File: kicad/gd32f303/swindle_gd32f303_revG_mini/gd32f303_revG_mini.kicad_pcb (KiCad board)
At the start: 2 copper layers, 39.3 x 30.1 mm, 54 parts, among them J1 Debug port, J2 Debug port, J3 USB, J40 J40, J7 Conn_01x05_Pin, Q1 DMG2302U, U1 GD32F303, U5 LM1117-3.3, Y2 8Mhz

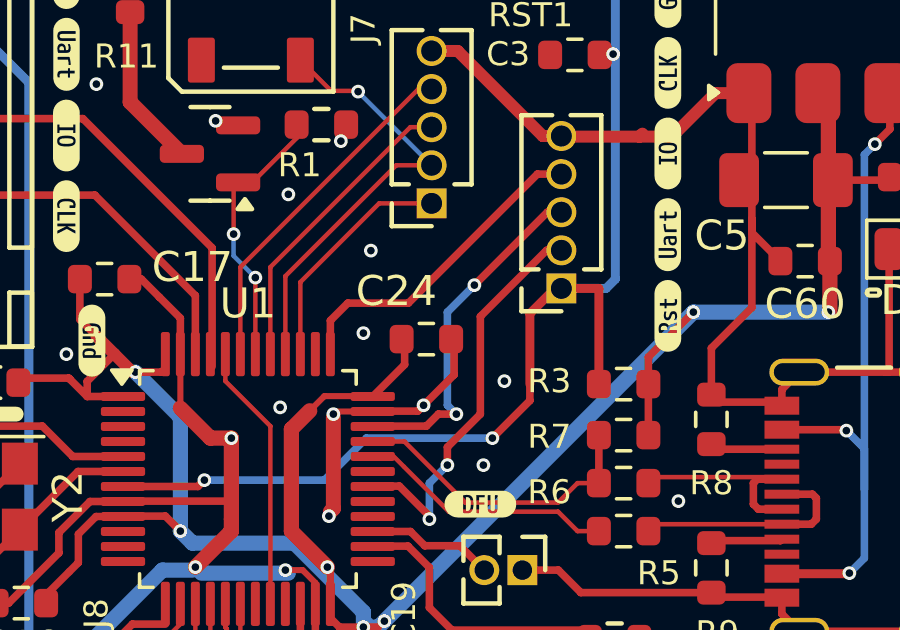
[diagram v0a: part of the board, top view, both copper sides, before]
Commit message: kicad : g32, cosmetic
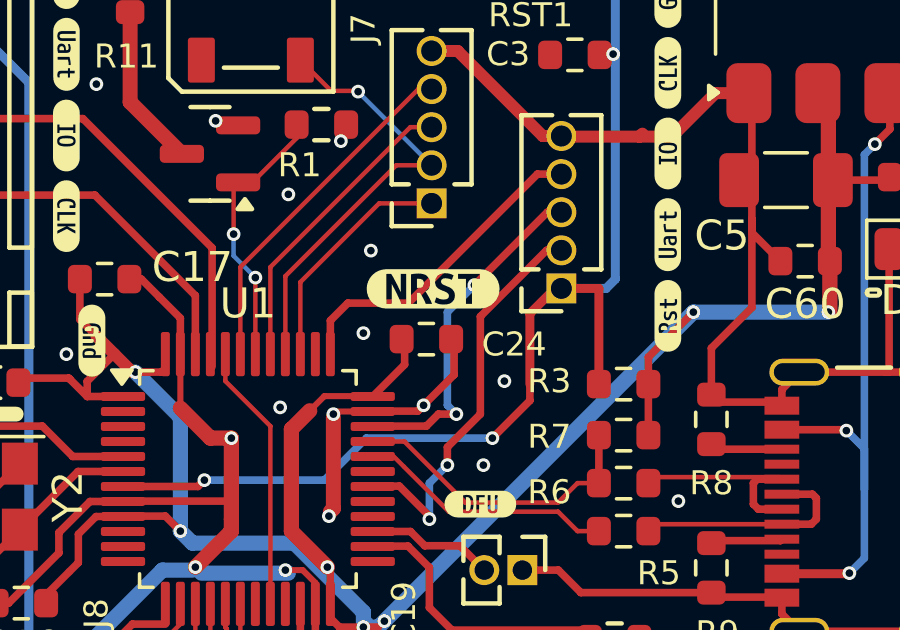
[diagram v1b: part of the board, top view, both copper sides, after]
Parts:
- added kibuzzard-68AB27BD: G***, kibuzzard-68AB27BD, F.Cu at (136.4, 84.6)
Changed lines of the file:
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@@
+		)
+	)
+	(footprint "kibuzzard-68AB27BD"
+		(layer "F.Cu")
+		(at 136.425 84.625)
+		(descr "Generated with KiBuzzard")
+		(tags "kb_params=eyJBbGlnbm1lbnRDaG9pY2UiOiAiQ2VudGVyIiwgIkNhcExlZnRDaG9pY2UiOiAiKCIsICJDYXBSaWdodENob2ljZSI6ICIpIiwgIkZvbnRDb21ib0JveCI6ICJVYnVudHVNb25vLUIiLCAiSGVpZ2h0Q3RybCI6IDEuMCwgIkxheWVyQ29tYm9Cb3giOiAiRi5TaWxrUyIsICJMaW5lU3BhY2luZ0N0cmwiOiAwLjYsICJNdWx0aUxpbmVUZXh0IjogIk5SU1QiLCAiUGFkZGluZ0JvdHRvbUN0cmwiOiAxLjAsICJQYWRkaW5nTGVmdEN0cmwiOiAwLjAsICJQYWRkaW5nUmlnaHRDdHJsIjogMC4wLCAiUGFkZGluZ1RvcEN0cmwiOiAxLjAsICJXaWR0aEN0cmwiOiAyLjgsICJhZHZhbmNlZENoZWNrYm94IjogZmFsc2UsICJpbmxpbmVGb3JtYXRUZXh0Ym94IjogZmFsc2UsICJsaW5lb3ZlclN0eWxlQ2hvaWNlIjogIlNxdWFyZSIsICJsaW5lb3ZlclRoaWNrbmVzc0N0cmwiOiAxfQ==")
+		(property "Reference" "kibuzzard-68AB27BD"
+			(at 0 -3.704435 0)
+			(layer "F.SilkS")
+			(hide yes)
+			(effects
+				(font
+					(size 0.001 0.001)
+				)
+			)
+		)
+		(property "Value" "G***"
+			(at 0 3.704435 0)
+			(layer "F.SilkS")
+			(hide yes)
+			(effects
+				(font
+					(size 0.001 0.001)
+				)
+			)
+		)
+		(property "Footprint" ""
+			(at 0 0 0)
+			(layer "F.Fab")
+			(hide yes)
+			(effects
+				(font
+					(size 1.27 1.27)
+					(thickness 0.15)
+				)
+			)
+		)
+		(property "Datasheet" ""
+			(at 0 0 0)
+			(layer "F.Fab")
+			(hide yes)
+			(effects
+				(font
+					(size 1.27 1.27)
+					(thickness 0.15)
+				)
+			)
+		)
+		(property "Description" ""
+			(at 0 0 0)
+			(layer "F.Fab")
+			(hide yes)
+			(effects
+				(font
+					(size 1.27 1.27)
+					(thickness 0.15)
+				)
+			)
+		)
+		(attr board_only exclude_from_pos_files exclude_from_bom)
+		(fp_poly
+			(pts
+				(xy -0.302908 -0.184168) (xy -0.315024 -0.252827) (xy -0.351373 -0.300485) (xy -0.407512 -0.328352)
+				(xy -0.478998 -0.337641) (xy -0.506462 -0.336834) (xy -0.538772 -0.332795) (xy -0.538772 -0.03231)
+				(xy -0.495153 -0.03231) (xy -0.407512 -0.042205) (xy -0.348142 -0.07189) (xy -0.302908 -0.184168)
+			)
+			(stroke
+				(width 0)
+				(type solid)
+			)
+			(fill solid)
+			(layer "F.SilkS")
+		)
+		(fp_poly
+			(pts
+				(xy -1.558158 -0.656435) (xy -1.558293 -0.656435) (xy -1.686357 -0.643822) (xy -1.8095 -0.606467)
+				(xy -1.922989 -0.545806) (xy -2.022463 -0.46417) (xy -2.104099 -0.364696) (xy -2.16476 -0.251207)
+				(xy -2.202115 -0.128064) (xy -2.214728 0) (xy -2.202115 0.128064) (xy -2.16476 0.251207) (xy -2.104099 0.364696)
+				(xy -2.022463 0.46417) (xy -1.922989 0.545806) (xy -1.8095 0.606467) (xy -1.686357 0.643822) (xy -1.558293 0.656435)
+				(xy -1.558158 0.656435) (xy -1.058966 0.656435) (xy -1.058966 0.500808) (xy -1.105547 0.389966)
+				(xy -1.15482 0.279304) (xy -1.206785 0.168821) (xy -1.261443 0.058338) (xy -1.318794 -0.052325)
+				(xy -1.378837 -0.163166) (xy -1.378837 0.500808) (xy -1.558158 0.500808) (xy -1.558158 -0.499192)
+				(xy -1.398223 -0.499192) (xy -1.352989 -0.425081) (xy -1.307754 -0.344911) (xy -1.263126 -0.261914)
+				(xy -1.219709 -0.179321) (xy -1.178514 -0.098142) (xy -1.140549 -0.019386) (xy -1.106826 0.053312)
+				(xy -1.078352 0.116317) (xy -1.078352 -0.499192) (xy -0.899031 -0.499192) (xy -0.899031 0.500808)
+				(xy -1.058966 0.500808) (xy -1.058966 0.656435) (xy -0.034733 0.656435) (xy -0.034733 0.500808)
+				(xy -0.243134 0.500808) (xy -0.28332 0.405695) (xy -0.329564 0.314216) (xy -0.380654 0.22395) (xy -0.43538 0.132472)
+				(xy -0.538772 0.132472) (xy -0.538772 0.500808) (xy -0.73748 0.500808) (xy -0.73748 -0.484653) (xy -0.673667 -0.496769)
+				(xy -0.603393 -0.504847) (xy -0.535541 -0.508885) (xy -0.478998 -0.510501) (xy -0.397415 -0.505654)
+				(xy -0.32391 -0.491115) (xy -0.259289 -0.466478) (xy -0.204362 -0.431341) (xy -0.127625 -0.328756)
+				(xy -0.107633 -0.261107) (xy -0.100969 -0.182553) (xy -0.109855 -0.099354) (xy -0.13651 -0.024233)
+				(xy -0.183764 0.038368) (xy -0.254443 0.084006) (xy -0.196284 0.176898) (xy -0.13651 0.283522) (xy -0.080775 0.394992)
+				(xy -0.034733 0.500808) (xy -0.034733 0.656435) (xy 0.357835 0.656435) (xy 0.357835 0.521809) (xy 0.245961 0.515145)
+				(xy 0.159128 0.495153) (xy 0.047658 0.44588) (xy 0.105816 0.28433) (xy 0.210016 0.332795) (xy 0.277262 0.349758)
+				(xy 0.357835 0.355412) (xy 0.441034 0.344911) (xy 0.493538 0.315832) (xy 0.520194 0.273829) (xy 0.527464 0.226171)
+				(xy 0.509693 0.171244) (xy 0.464459 0.128433) (xy 0.403069 0.094507) (xy 0.335218 0.066236) (xy 0.241519 0.029079)
+				(xy 0.153473 -0.024233) (xy 0.088045 -0.1042) (xy 0.062197 -0.22294) (xy 0.085016 -0.348142) (xy 0.153473 -0.442649)
+				(xy 0.221953 -0.486627) (xy 0.30569 -0.513014) (xy 0.404685 -0.521809) (xy 0.490913 -0.516559) (xy 0.565428 -0.500808)
+				(xy 0.680937 -0.453958) (xy 0.622779 -0.300485) (xy 0.533118 -0.339257) (xy 0.419225 -0.355412)
+				(xy 0.331269 -0.342667) (xy 0.278496 -0.304434) (xy 0.260905 -0.240711) (xy 0.27706 -0.189822) (xy 0.318255 -0.15105)
+				(xy 0.374798 -0.121163) (xy 0.436995 -0.096931) (xy 0.534733 -0.057351) (xy 0.628433 0.000808) (xy 0.698708 0.091276)
+				(xy 0.719305 0.152464) (xy 0.726171 0.227787) (xy 0.703352 0.352383) (xy 0.634895 0.445073) (xy 0.563543 0.487704)
+				(xy 0.47119 0.513283) (xy 0.357835 0.521809) (xy 0.357835 0.656435) (xy 1.29483 0.656435) (xy 1.29483 0.500808)
+				(xy 1.094507 0.500808) (xy 1.094507 -0.33441) (xy 0.831179 -0.33441) (xy 0.831179 -0.499192) (xy 1.558158 -0.499192)
+				(xy 1.558158 -0.33441) (xy 1.29483 -0.33441) (xy 1.29483 0.500808) (xy 1.29483 0.656435) (xy 1.558158 0.656435)
+				(xy 1.558293 0.656435) (xy 1.686357 0.643822) (xy 1.8095 0.606467) (xy 1.922989 0.545806) (xy 2.022463 0.46417)
+				(xy 2.104099 0.364696) (xy 2.16476 0.251207) (xy 2.202115 0.128064) (xy 2.214728 0) (xy 2.202115 -0.128064)
+				(xy 2.16476 -0.251207) (xy 2.104099 -0.364696) (xy 2.022463 -0.46417) (xy 1.922989 -0.545806) (xy 1.8095 -0.606467)
+				(xy 1.686357 -0.643822) (xy 1.558293 -0.656435) (xy 1.558158 -0.656435) (xy -1.558158 -0.656435)
+			)
+			(stroke
+				(width 0)
+				(type solid)
+			)
+			(fill solid)
+			(layer "F.SilkS")
 		)
 	)
@@
 		(tags "resistor")
 		(property "Reference" "C24"
-			(at -1 -1.6 0)
-			(layer "F.SilkS")
-			(effects
-				(font
-					(size 1 1)
-					(thickness 0.15)
-				)
+			(at 2.925 0.175 0)
+			(layer "F.SilkS")
+			(effects
+				(font
+					(size 0.8 0.8)
+					(thickness 0.15)
+				)
